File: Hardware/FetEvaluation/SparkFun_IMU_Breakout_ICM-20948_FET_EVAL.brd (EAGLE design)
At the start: 31.8 x 25.4 mm, 118 parts, among them Q1 DMN2005LP4K-7, Q10 RE1C002UN, Q11 DMN2005LP4K-7, Q12 RE1C002UN, Q13 DMN2005LP4K-7, Q14 RE1C002UN, Q15 DMN2005LP4K-7, Q16 RE1C002UN, Q2 RE1C002UN, Q3 DMN2005LP4K-7, Q4 RE1C002UN, Q5 DMN2005LP4K-7, Q6 RE1C002UN, Q7 DMN2005LP4K-7, Q8 RE1C002UN, Q9 DMN2005LP4K-7, U1 TP, U10 TP, U11 TP, U12 TP, U13 TP, U14 TP, U15 TP, U16 TP, U17 TP, U18 TP, U2 9DoF IMU, U3 1.8V/100mA, U4 TP, U5 TP, U6 TP, U7 TP, U8 TP, U9 TP

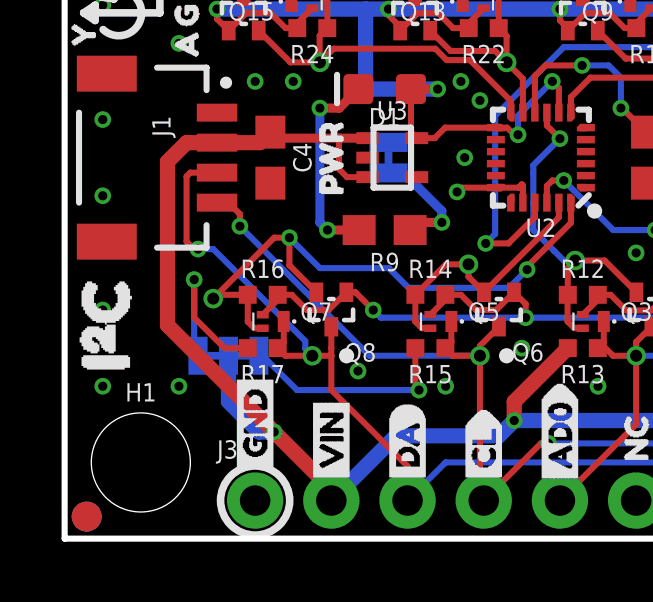
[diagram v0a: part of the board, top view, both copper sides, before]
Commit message: Commit for design review
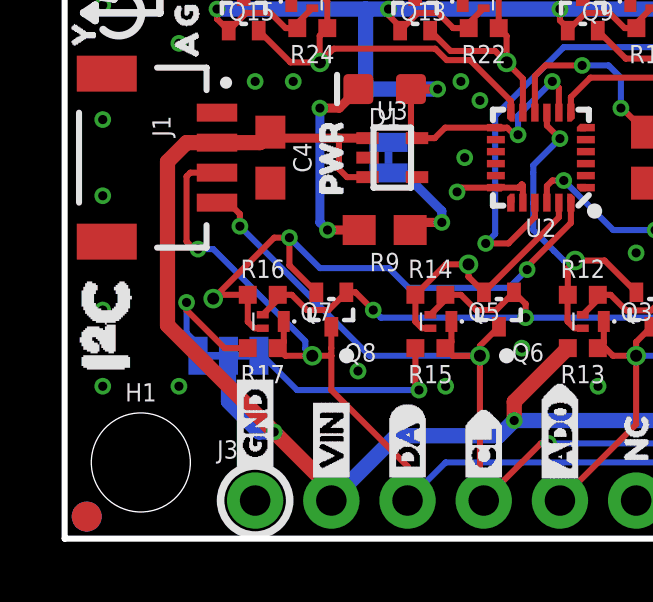
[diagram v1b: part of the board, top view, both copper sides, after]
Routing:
- net SDA/SDI_VIN_JMP: track 6.07 -> 4.76 mm
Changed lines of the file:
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@@
 <contactref element="R17" pad="2"/>
 <contactref element="JP4" pad="1"/>
-<wire x1="4.318" y1="7.366" x2="5.334" y2="6.35" width="0.2032" layer="1"/>
-<via x="4.318" y="8.636" extent="1-16" drill="0.3048"/>
-<wire x1="4.318" y1="8.636" x2="4.318" y2="6.223" width="0.2032" layer="16"/>
-<wire x1="4.318" y1="8.636" x2="4.318" y2="7.366" width="0.2032" layer="1"/>
+<wire x1="4.064" y1="7.62" x2="5.334" y2="6.35" width="0.2032" layer="1"/>
+<via x="4.064" y="7.874" extent="1-16" drill="0.3048"/>
+<wire x1="4.064" y1="7.874" x2="4.064" y2="6.858" width="0.2032" layer="16"/>
+<wire x1="4.064" y1="7.874" x2="4.064" y2="7.62" width="0.2032" layer="1"/>
 <wire x1="5.334" y1="6.35" x2="6.104" y2="6.35" width="0.2032" layer="1"/>
-<wire x1="4.318" y1="6.223" x2="4.445" y2="6.096" width="0.2032" layer="16"/>
+<wire x1="4.064" y1="6.858" x2="4.445" y2="6.477" width="0.2032" layer="16"/>
+<wire x1="4.445" y1="6.477" x2="4.445" y2="6.096" width="0.2032" layer="16"/>
 </signal>
 <signal name="SCL/SCLK_VIN_JMP">
